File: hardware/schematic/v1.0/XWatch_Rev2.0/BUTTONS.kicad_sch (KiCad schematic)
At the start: 5 parts, among them SW1 EVPAEDB2A, SW2 EVPAEDB2A, SW3 EVPAEDB2A, SW4 EVPAEDB2A, SW5 EVPAEDB2A

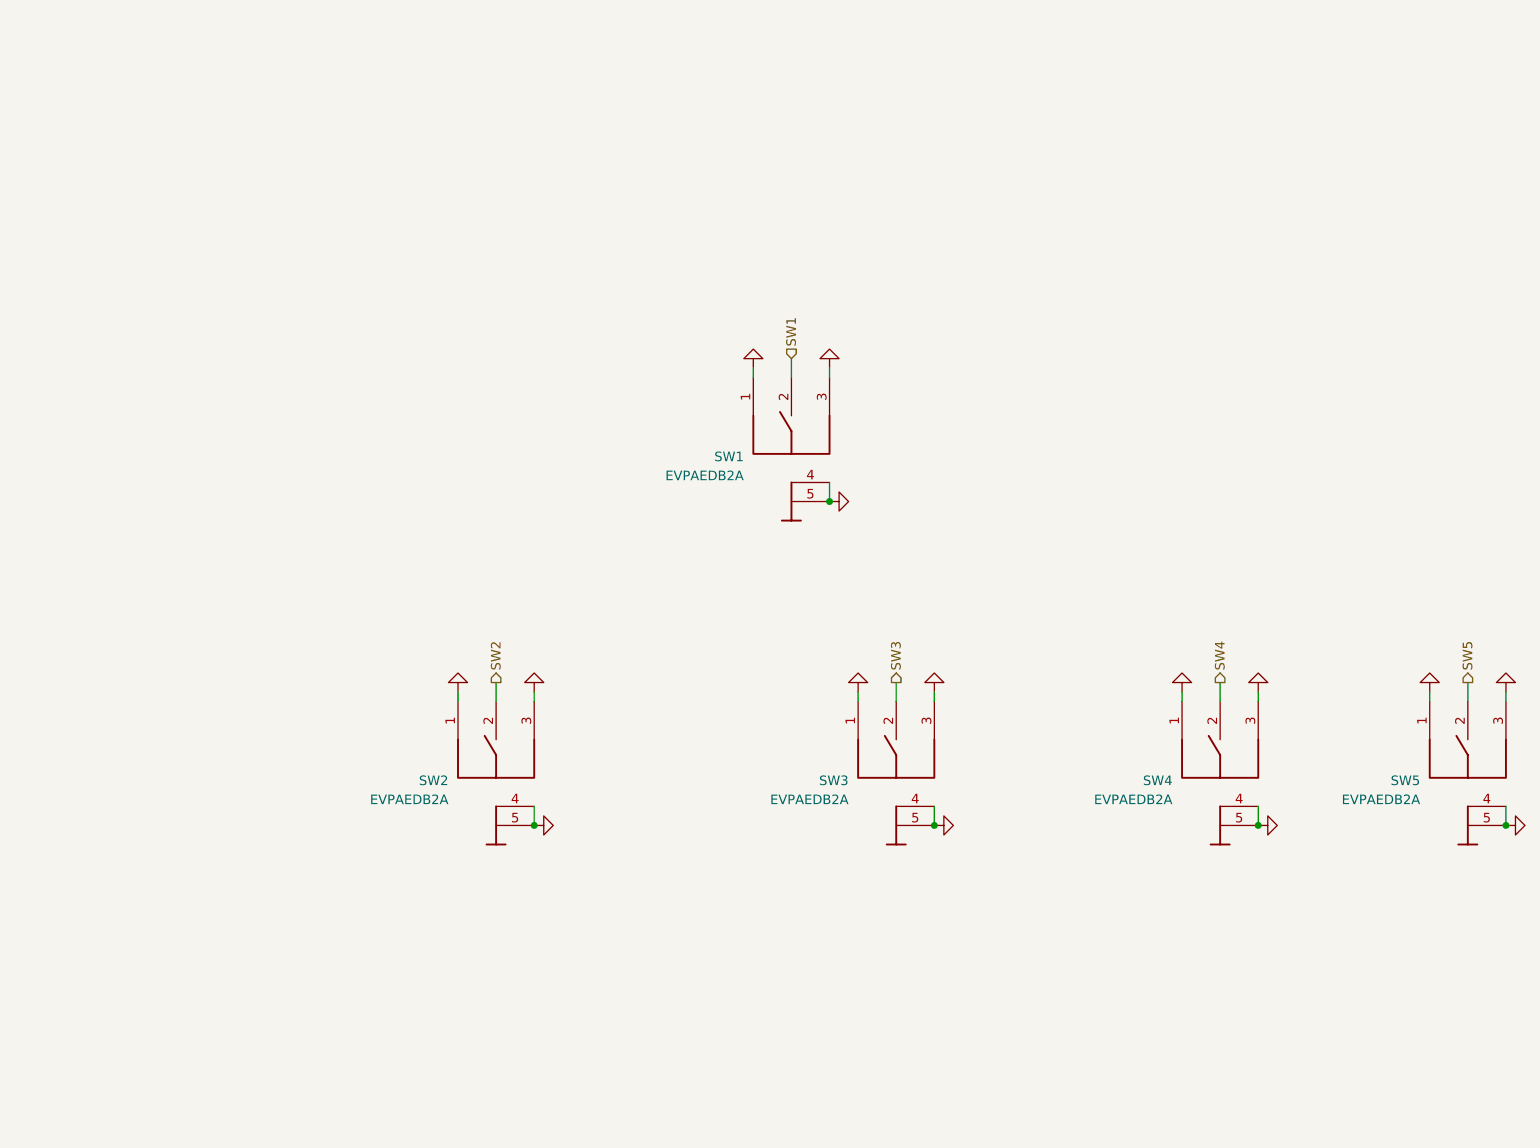
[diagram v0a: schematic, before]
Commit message: sch update
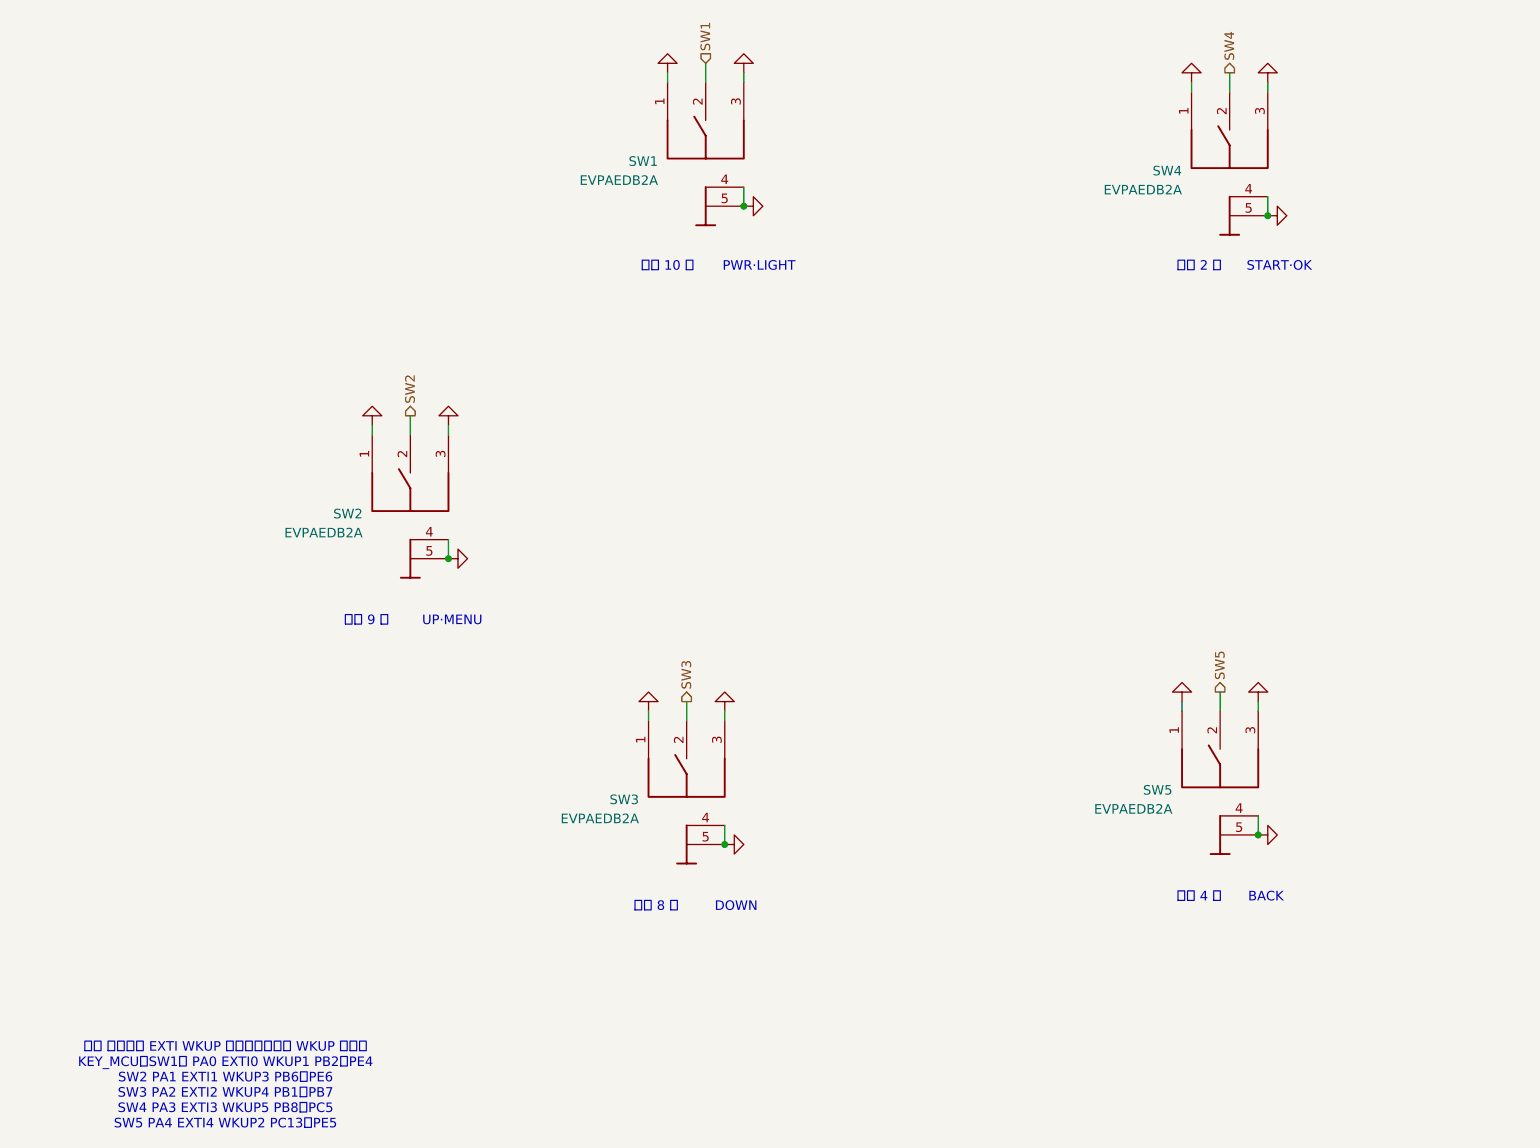
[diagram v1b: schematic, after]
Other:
- note added: "BACK"
- note added: "DOWN"
- note added: "PWR·LIGHT"
- note added: "START·OK"
- note added: "UP·MENU"
- note added: "右上 2 点"
- note added: "右下 4 点"
- note added: "左上 10 点"
- note added: "左下 8 点"
- note added: "左中 9 点"
- note added: "网络 建议引脚 EXTI WKUP 备选引脚（同一 WKUP 编号） KEY_MCU（SW1） PA0 EXTI0 WKUP1 PB2、PE4 SW2 PA1 EXTI1 WKUP3 PB6、PE6 SW3 PA2 EXTI2 WKUP4 PB1、PB7 SW4 PA3 EXTI3 WKUP5 PB8、PC5 SW5 PA4 EXTI4 WKUP2 PC13、PE5"
- moved on the sheet: SW1, SW2, SW3, SW4, SW5

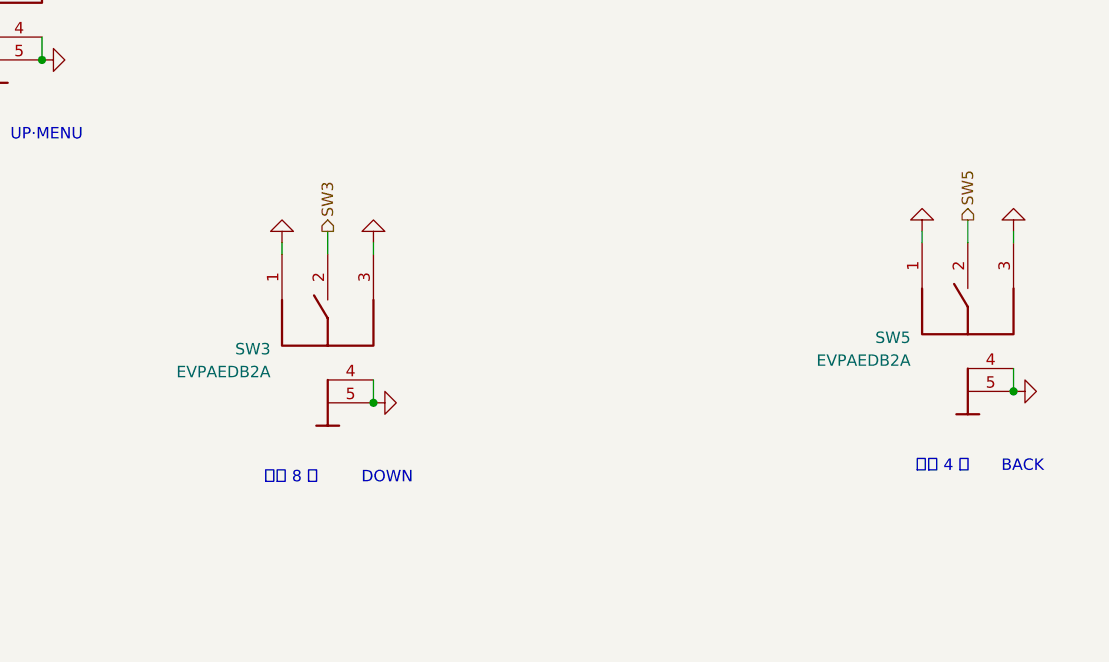
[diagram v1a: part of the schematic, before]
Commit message: sch update
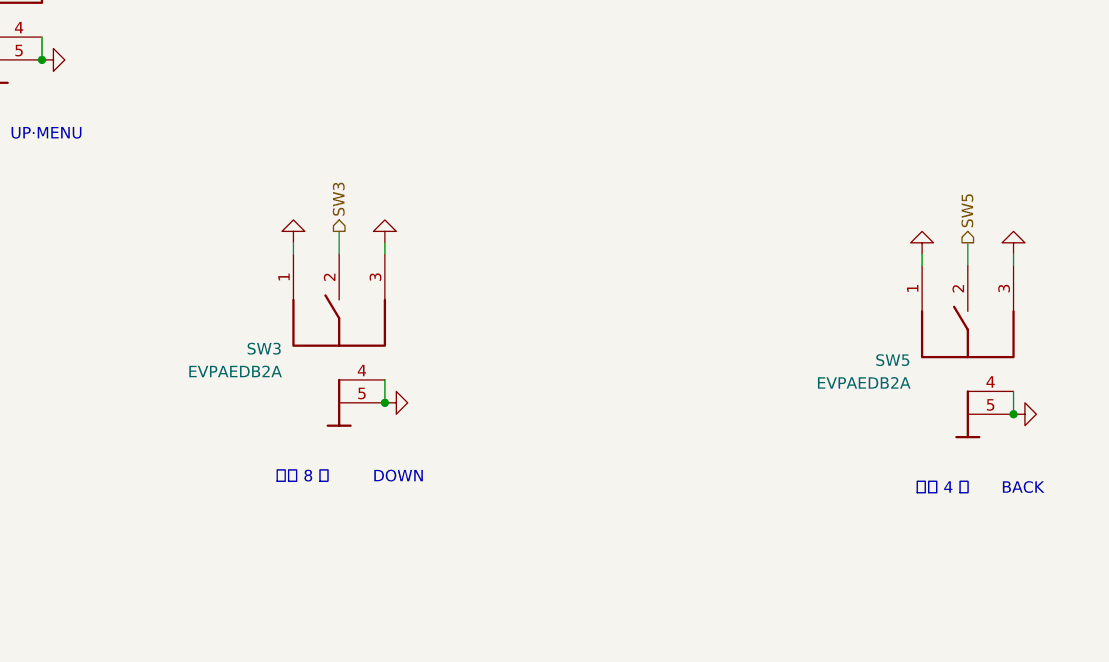
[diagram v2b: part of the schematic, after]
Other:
- moved on the sheet: SW3, SW5
